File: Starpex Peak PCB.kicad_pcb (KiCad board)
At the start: 2 copper layers, 83.2 x 59.7 mm, 5 parts, among them J1 Conn_01x12_Pin, J2 Conn_01x20_Pin, SW1 SW_SPDT_321, SW2 SW_Push, SW3 SW_Push

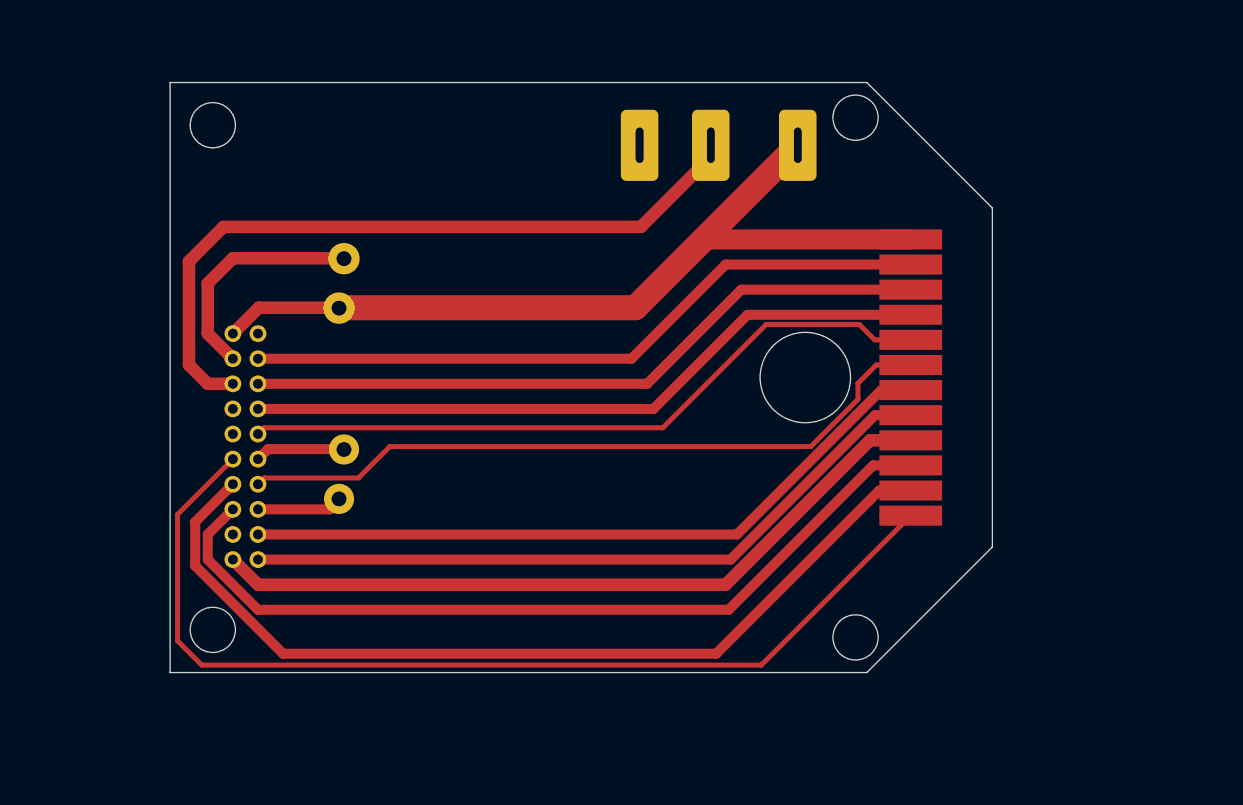
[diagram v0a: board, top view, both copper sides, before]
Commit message: help from Vincent Santosa
with the old DuPont connector design
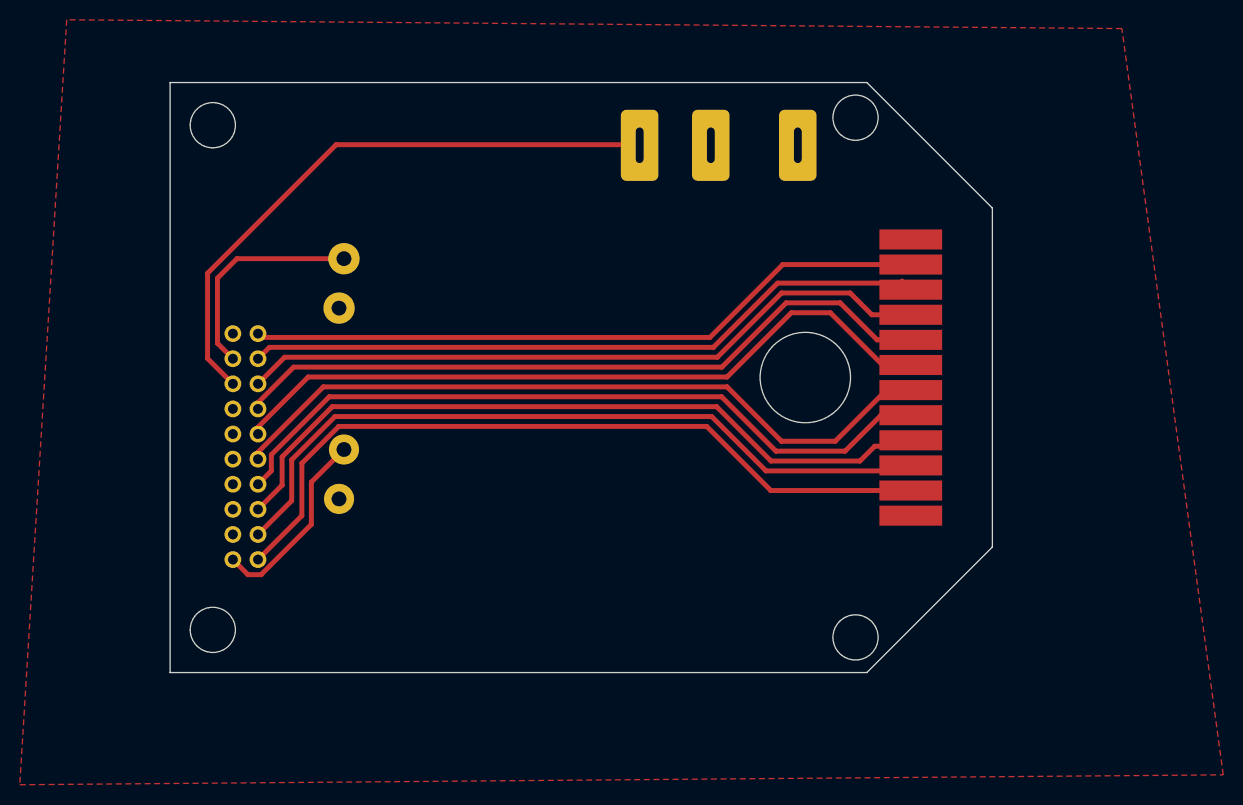
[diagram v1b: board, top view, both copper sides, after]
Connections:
- net Net-(J2-Pin_4) renamed /B2
- J1 pad 1: Net-(J1-Pin_1) -> /GND
- J1 pad 10: Net-(J1-Pin_10) -> /9
- J1 pad 11: Net-(J1-Pin_11) -> /10
- J1 pad 12: Net-(J1-Pin_12) -> /GND
- J1 pad 2: Net-(J1-Pin_2) -> /1
- J1 pad 3: Net-(J1-Pin_3) -> /2
- J1 pad 4: Net-(J1-Pin_4) -> /3
- J1 pad 5: Net-(J1-Pin_5) -> /4
- J1 pad 6: Net-(J1-Pin_6) -> /5
- J1 pad 7: Net-(J1-Pin_7) -> /6
- J1 pad 8: Net-(J1-Pin_8) -> /7
- J1 pad 9: Net-(J1-Pin_9) -> /8
- J2 pad 1: unconnected-(J2-Pin_1-Pad1) -> /1
- J2 pad 11: Net-(J2-Pin_11) -> /6
- J2 pad 12: Net-(J1-Pin_12) -> unconnected-(J2-Pin_12-Pad12)
- J2 pad 13: Net-(J1-Pin_6) -> /7
- J2 pad 14: Net-(J1-Pin_11) -> unconnected-(J2-Pin_14-Pad14)
- J2 pad 15: Net-(J2-Pin_15) -> /8
- J2 pad 16: Net-(J1-Pin_10) -> unconnected-(J2-Pin_16-Pad16)
- J2 pad 17: Net-(J1-Pin_7) -> /9
- J2 pad 19: Net-(J1-Pin_8) -> /10
- J2 pad 2: Net-(J1-Pin_1) -> /GND
- J2 pad 20: Net-(J1-Pin_9) -> /B1
- J2 pad 3: Net-(J1-Pin_2) -> /2
- J2 pad 5: Net-(J1-Pin_3) -> /3
- J2 pad 6: Net-(J2-Pin_6) -> /B3
- J2 pad 7: Net-(J1-Pin_4) -> /4
- J2 pad 9: Net-(J1-Pin_5) -> /5
- SW1 pad 1: Net-(J1-Pin_1) -> unconnected-(SW1-C-Pad1)
- SW1 pad 2: Net-(J2-Pin_6) -> /GND
- SW1 pad 3: unconnected-(SW1-A-Pad3) -> /B3
- SW2 pad 2: Net-(J1-Pin_1) -> /GND
- SW3 pad 1: Net-(J2-Pin_11) -> /B1
- SW3 pad 2: Net-(J2-Pin_15) -> /GND
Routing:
- net Net-(J1-Pin_12): track 104.7 -> 0.00 mm
- net Net-(J1-Pin_11): track 92.7 -> 0.00 mm
- net Net-(J1-Pin_1): track 86.0 -> 0.00 mm
- net Net-(J1-Pin_10): track 85.4 -> 0.00 mm
- net /10: track 0.00 -> 77.4 mm
- net /9: track 0.00 -> 75.9 mm
- net Net-(J1-Pin_9): track 75.7 -> 0.00 mm
- net /8: track 0.00 -> 75.2 mm
- net /7: track 0.00 -> 74.5 mm
- net Net-(J2-Pin_6): track 74.1 -> 0.00 mm
- net /6: track 0.00 -> 73.9 mm
- net /5: track 0.00 -> 73.7 mm
- net /4: track 0.00 -> 72.4 mm
- net Net-(J1-Pin_6): track 72.2 -> 0.00 mm
- net Net-(J1-Pin_8): track 72.1 -> 0.00 mm
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- added copper zone on F.Cu, net /GND
